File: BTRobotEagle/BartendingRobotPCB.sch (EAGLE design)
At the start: 44 parts, among them P1 B2B-XH-A(LF)(SN), P10 B2B-XH-A(LF)(SN), P11 B2B-XH-A(LF)(SN), P2 B2B-XH-A(LF)(SN), P3 B2B-XH-A(LF)(SN), P4 B2B-XH-A(LF)(SN), P5 B2B-XH-A(LF)(SN), P6 B2B-XH-A(LF)(SN), P7 B2B-XH-A(LF)(SN), P8 B2B-XH-A(LF)(SN), P9 B2B-XH-A(LF)(SN)

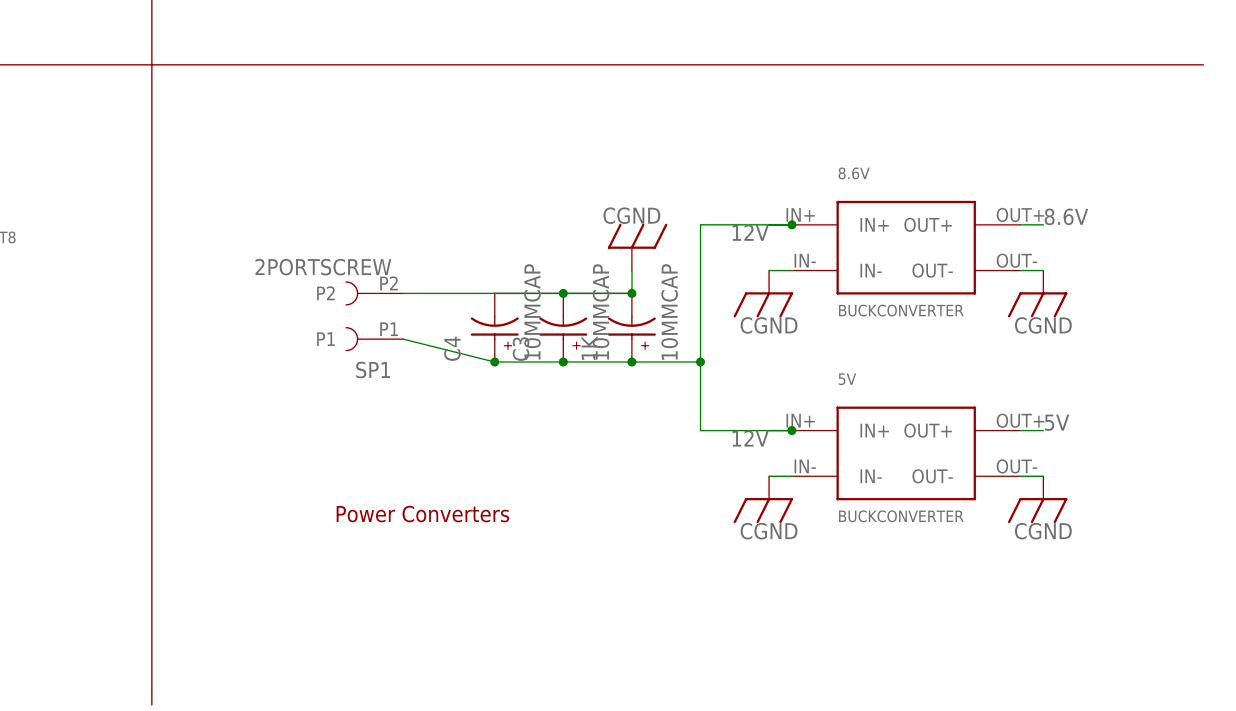
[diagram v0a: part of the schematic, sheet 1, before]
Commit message: more changes
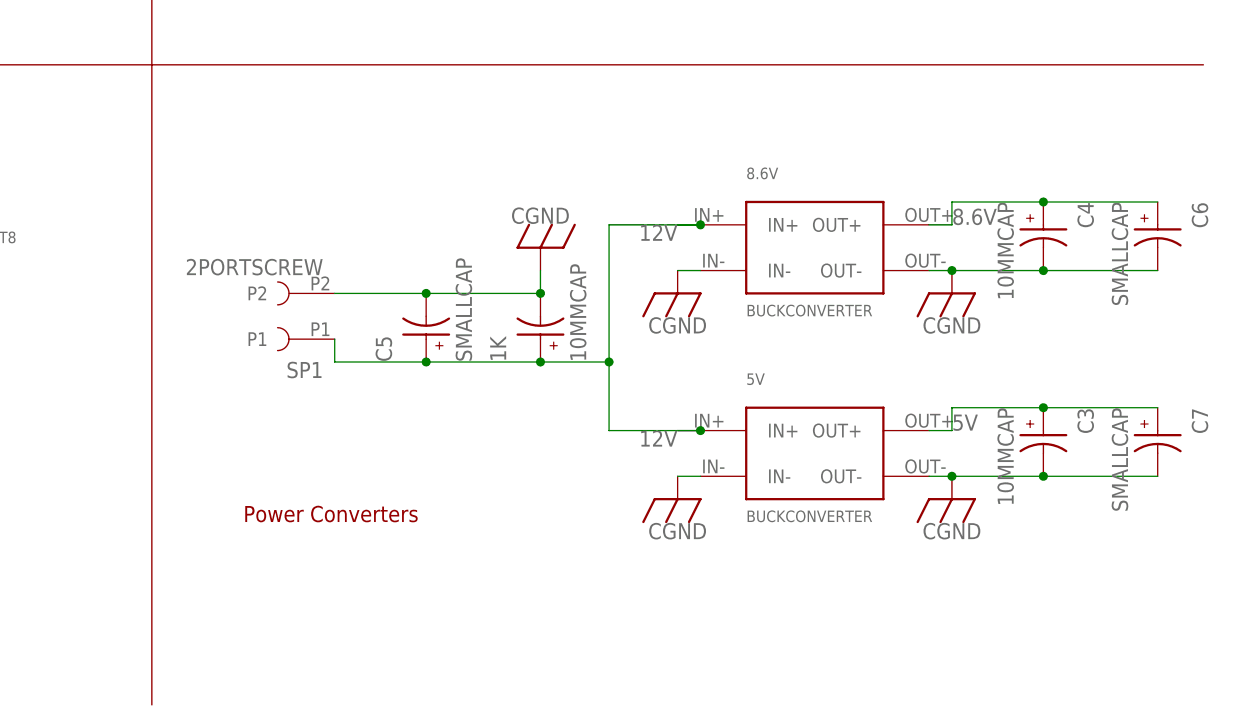
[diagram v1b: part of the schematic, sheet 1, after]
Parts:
- added C5, C6, C7: SMALLCAP, BartendingRobot:SMALLCAP
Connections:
- net 12V: now also C5.P; no longer C3.P, C4.P
- net 5V: now also C3.P, C7.P
- net 8.6V: now also C4.P, C6.P
- net CGND: now also C5.N, C6.N, C7.N
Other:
- moved on the sheet: 1K, 5V, 8.6V, C3, C4, SP1
